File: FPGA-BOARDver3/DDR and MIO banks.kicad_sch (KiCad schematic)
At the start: 1 part, among them U1 XC7Z020-1CLG400I__

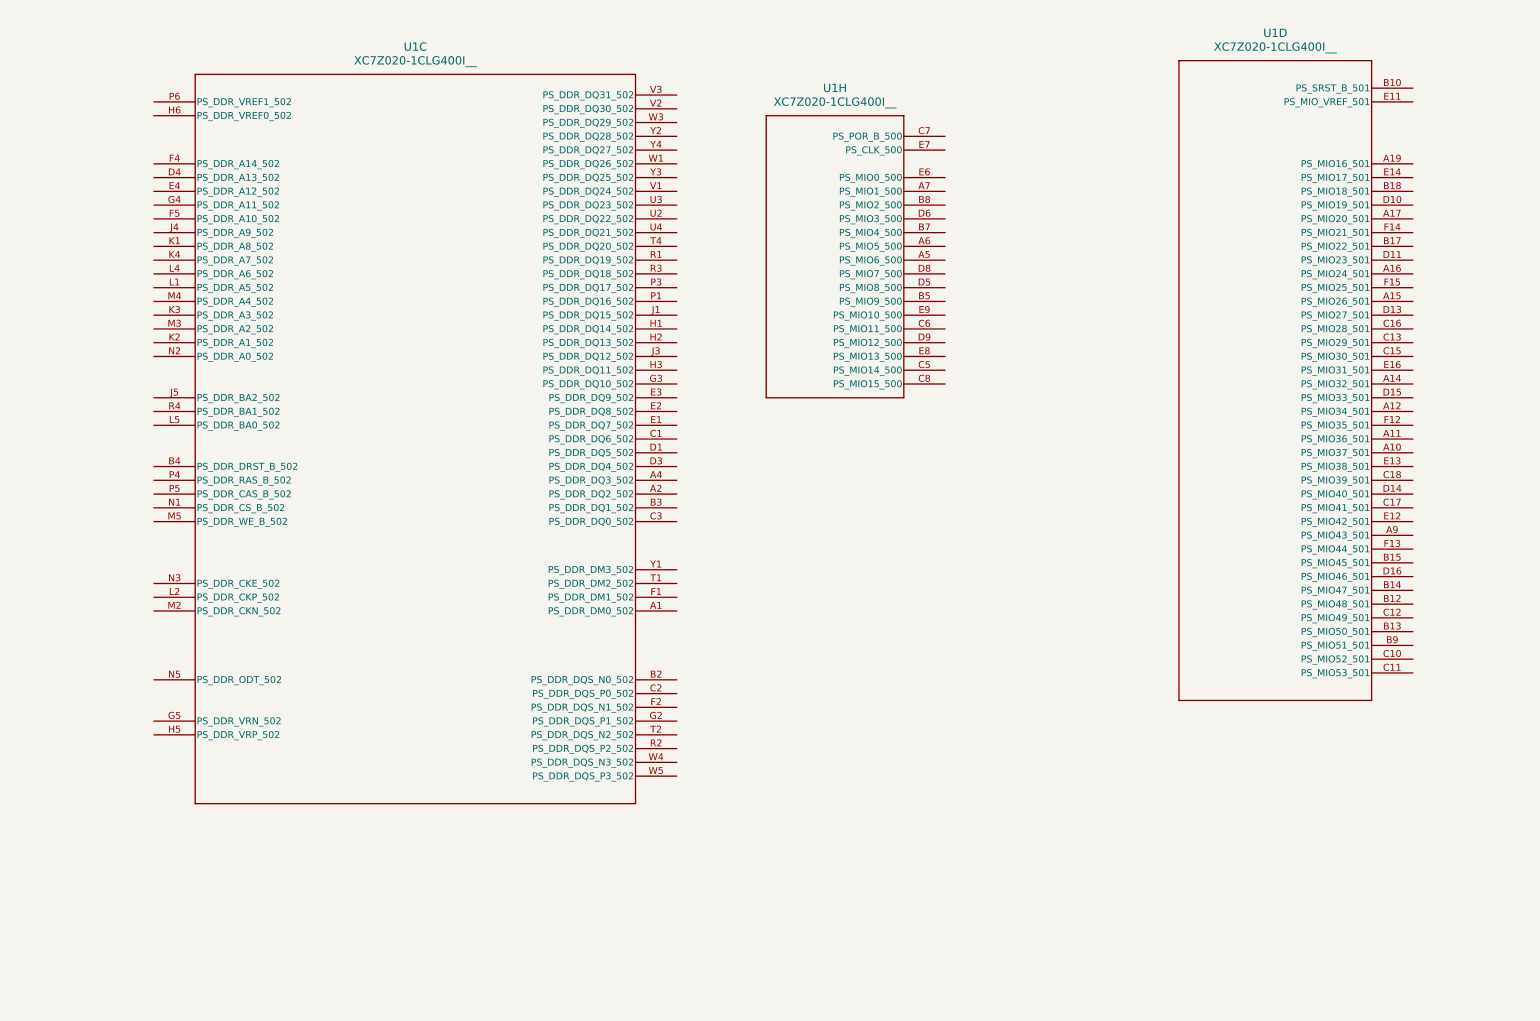
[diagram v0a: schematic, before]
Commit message: spdif fpga bansks
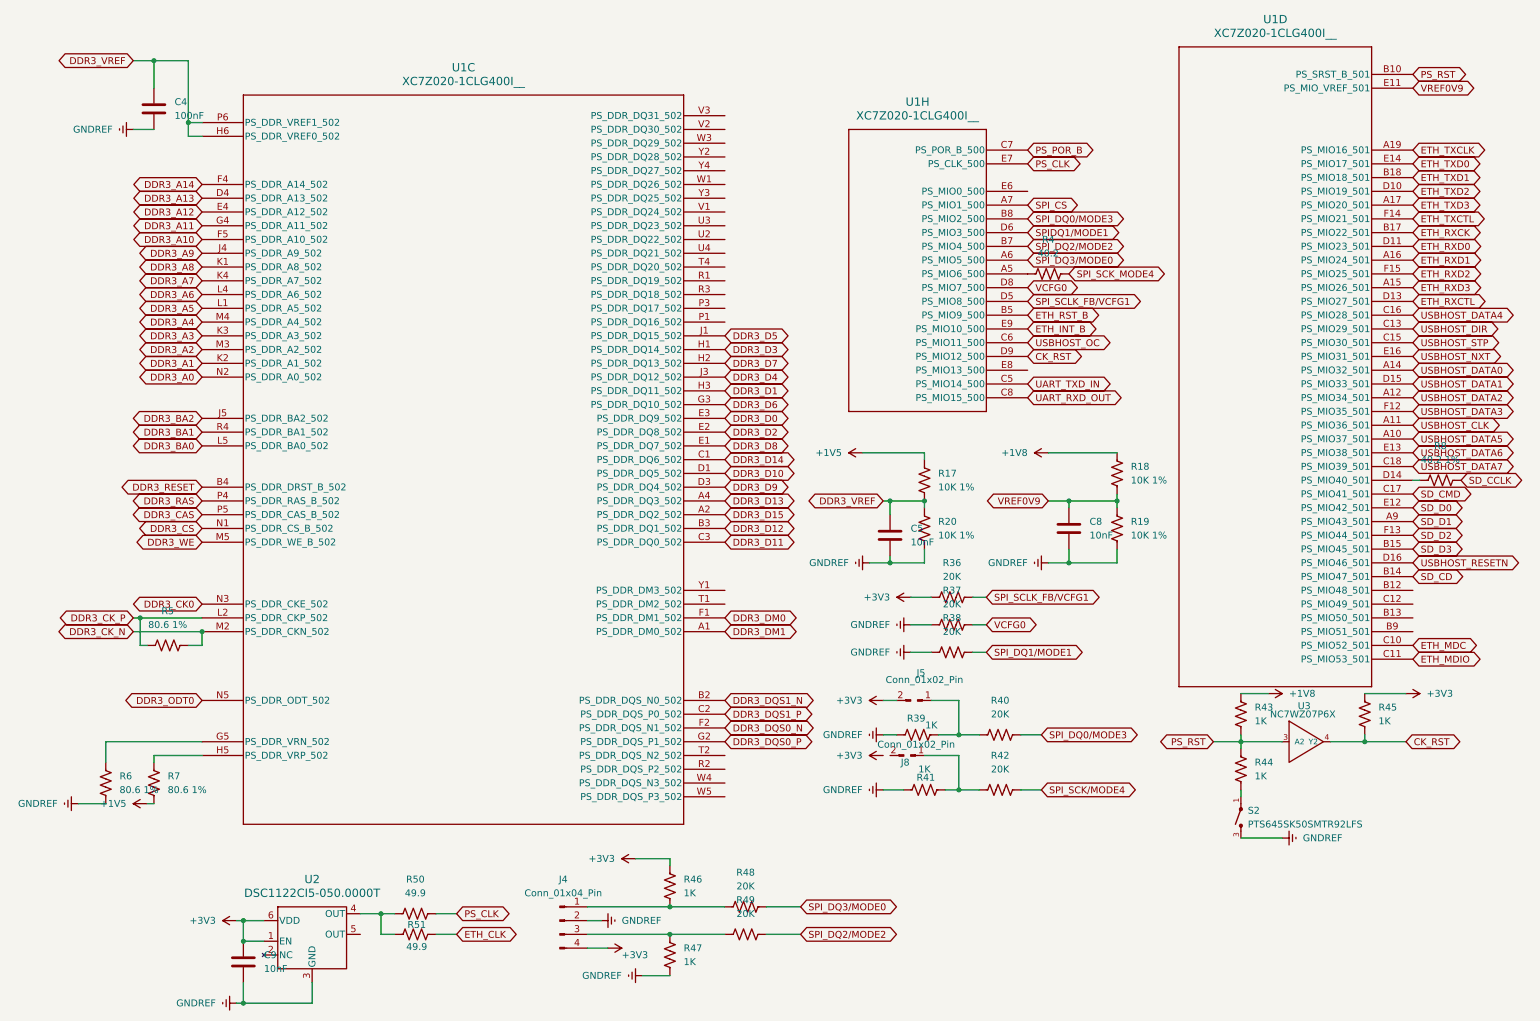
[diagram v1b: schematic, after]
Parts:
- added C4: 100nF, footprints:C_0402, symbol Device:C
- added C5, C8, C9: 10nF, footprints:C_0402, symbol Device:C
- added J4: Conn_01x04_Pin, footprints:CONN_PZ254V-11-04P_XFC, symbol Connector:Conn_01x04_Pin
- added J5, J8: Conn_01x02_Pin, footprints:CONN_PZ254V-11-02P_02P_XFC, symbol Connector:Conn_01x02_Pin
- added R17, R18, R19, R20: 10K 1%, footprints:R_0402, symbol Device:R_US
- added R36, R37, R38, R40, R42, R48, R49: 20K, footprints:R_0402, symbol Device:R_US
- added R39, R41, R43, R44, R45, R46, R47: 1K, footprints:R_0402, symbol Device:R_US
- added R4: 40.2, footprints:R_0402, symbol Device:R_US
- added R5, R6, R7: 80.6 1%, footprints:R_0402, symbol Device:R_US
- added R50, R51: 49.9, footprints:R_0402, symbol Device:R_US
- added R8: 40.2 1%, footprints:R_0402, symbol Device:R_US
- added S2: PTS645SK50SMTR92LFS, footprints:SW_PTS645SK50SMTR92LFS, symbol PTS645SK50SMTR92LFS:PTS645SK50SMTR92LFS
- added U2: DSC1122CI5-050.0000T, footprints:VDFN6_3P2X2P5_MCH, symbol 2025-04-06_19-32-54:DSC1122CI5-050.0000T
- added U3: NC7WZ07P6X, footprints:NC7WZ07P6X, symbol NC7WZ07P6X:NC7WZ07P6X
- U1: footprint footprints:CLG400_ZYNQ-7000_AMD -> XC7Z020-1CLG400I:CLG400_ZYNQ-7000_AMD
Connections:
- net DDR3_DM1: now reaches U1.A1 (PS_DDR_DM0_502)
- net DDR3_D15: now reaches U1.A2 (PS_DDR_DQ2_502)
- net DDR3_D13: now reaches U1.A4 (PS_DDR_DQ3_502)
- net DDR3_DQS1_N: now reaches U1.B2 (PS_DDR_DQS_N0_502)
- net DDR3_D12: now reaches U1.B3 (PS_DDR_DQ1_502)
- net DDR3_RESET: now reaches U1.B4 (PS_DDR_DRST_B_502)
- net DDR3_D14: now reaches U1.C1 (PS_DDR_DQ6_502)
- net DDR3_DQS1_P: now reaches U1.C2 (PS_DDR_DQS_P0_502)
- net DDR3_D11: now reaches U1.C3 (PS_DDR_DQ0_502)
- net DDR3_D10: now reaches U1.D1 (PS_DDR_DQ5_502)
- net DDR3_D9: now reaches U1.D3 (PS_DDR_DQ4_502)
- net DDR3_A13: now reaches U1.D4 (PS_DDR_A13_502)
- net DDR3_D8: now reaches U1.E1 (PS_DDR_DQ7_502)
- net DDR3_D2: now reaches U1.E2 (PS_DDR_DQ8_502)
- net DDR3_D0: now reaches U1.E3 (PS_DDR_DQ9_502)
- net DDR3_A12: now reaches U1.E4 (PS_DDR_A12_502)
- net DDR3_DM0: now reaches U1.F1 (PS_DDR_DM1_502)
- net DDR3_DQS0_N: now reaches U1.F2 (PS_DDR_DQS_N1_502)
- net DDR3_A14: now reaches U1.F4 (PS_DDR_A14_502)
- net DDR3_A10: now reaches U1.F5 (PS_DDR_A10_502)
- net DDR3_DQS0_P: now reaches U1.G2 (PS_DDR_DQS_P1_502)
- net DDR3_D6: now reaches U1.G3 (PS_DDR_DQ10_502)
- net DDR3_A11: now reaches U1.G4 (PS_DDR_A11_502)
- net at U1.G5 (PS_DDR_VRN_502): now also R6.2
- net DDR3_D3: now reaches U1.H1 (PS_DDR_DQ14_502)
- net DDR3_D7: now reaches U1.H2 (PS_DDR_DQ13_502)
- net DDR3_D1: now reaches U1.H3 (PS_DDR_DQ11_502)
- net at U1.H5 (PS_DDR_VRP_502): now also R7.2
- net DDR3_VREF: now reaches U1.H6 (PS_DDR_VREF0_502)
- net DDR3_VREF: now also U1.P6 (PS_DDR_VREF1_502), C4.1, C5.1, R17.2, R20.1
- net DDR3_D5: now reaches U1.J1 (PS_DDR_DQ15_502)
- net DDR3_D4: now reaches U1.J3 (PS_DDR_DQ12_502)
- net DDR3_A9: now reaches U1.J4 (PS_DDR_A9_502)
- net DDR3_BA2: now reaches U1.J5 (PS_DDR_BA2_502)
- net DDR3_A8: now reaches U1.K1 (PS_DDR_A8_502)
- net DDR3_A1: now reaches U1.K2 (PS_DDR_A1_502)
- net DDR3_A3: now reaches U1.K3 (PS_DDR_A3_502)
- net DDR3_A7: now reaches U1.K4 (PS_DDR_A7_502)
- net DDR3_A5: now reaches U1.L1 (PS_DDR_A5_502)
- net DDR3_CK_P: now reaches U1.L2 (PS_DDR_CKP_502)
- net DDR3_CK_P: now also R5.1
- net DDR3_A6: now reaches U1.L4 (PS_DDR_A6_502)
- net DDR3_BA0: now reaches U1.L5 (PS_DDR_BA0_502)
- net DDR3_CK_N: now reaches U1.M2 (PS_DDR_CKN_502)
- net DDR3_CK_N: now also R5.2
- net DDR3_A2: now reaches U1.M3 (PS_DDR_A2_502)
- net DDR3_A4: now reaches U1.M4 (PS_DDR_A4_502)
- net DDR3_WE: now reaches U1.M5 (PS_DDR_WE_B_502)
- net DDR3_CS: now reaches U1.N1 (PS_DDR_CS_B_502)
- net DDR3_A0: now reaches U1.N2 (PS_DDR_A0_502)
- net DDR3_CK0: now reaches U1.N3 (PS_DDR_CKE_502)
- net DDR3_ODT0: now reaches U1.N5 (PS_DDR_ODT_502)
- net DDR3_RAS: now reaches U1.P4 (PS_DDR_RAS_B_502)
- net DDR3_CAS: now reaches U1.P5 (PS_DDR_CAS_B_502)
- net DDR3_BA1: now reaches U1.R4 (PS_DDR_BA1_502)
- net USBHOST_DATA5: now reaches U1.A10 (PS_MIO37_501)
- net USBHOST_CLK: now reaches U1.A11 (PS_MIO36_501)
- net USBHOST_DATA2: now reaches U1.A12 (PS_MIO34_501)
- net USBHOST_DATA0: now reaches U1.A14 (PS_MIO32_501)
- net ETH_RXD3: now reaches U1.A15 (PS_MIO26_501)
- net ETH_RXD1: now reaches U1.A16 (PS_MIO24_501)
- net ETH_TXD3: now reaches U1.A17 (PS_MIO20_501)
- net ETH_TXCLK: now reaches U1.A19 (PS_MIO16_501)
- net SD_D1: now reaches U1.A9 (PS_MIO43_501)
- net PS_RST: now reaches U1.B10 (PS_SRST_B_501)
- net PS_RST: now also R43.2, R44.2, U3.3 (A2)
- net SD_CD: now reaches U1.B14 (PS_MIO47_501)
- net SD_D3: now reaches U1.B15 (PS_MIO45_501)
- net ETH_RXCK: now reaches U1.B17 (PS_MIO22_501)
- net ETH_TXD1: now reaches U1.B18 (PS_MIO18_501)
- net ETH_MDC: now reaches U1.C10 (PS_MIO52_501)
- net ETH_MDIO: now reaches U1.C11 (PS_MIO53_501)
- net USBHOST_DIR: now reaches U1.C13 (PS_MIO29_501)
- net USBHOST_STP: now reaches U1.C15 (PS_MIO30_501)
- net USBHOST_DATA4: now reaches U1.C16 (PS_MIO28_501)
- net SD_CMD: now reaches U1.C17 (PS_MIO41_501)
- net USBHOST_DATA7: now reaches U1.C18 (PS_MIO39_501)
- net ETH_TXD2: now reaches U1.D10 (PS_MIO19_501)
- net ETH_RXD0: now reaches U1.D11 (PS_MIO23_501)
- net ETH_RXCTL: now reaches U1.D13 (PS_MIO27_501)
- net at U1.D14 (PS_MIO40_501): now also R8.1
- net USBHOST_DATA1: now reaches U1.D15 (PS_MIO33_501)
- net USBHOST_RESETN: now reaches U1.D16 (PS_MIO46_501)
- net VREF0V9: now reaches U1.E11 (PS_MIO_VREF_501)
- net VREF0V9: now also C8.1, R18.2, R19.1
- net SD_D0: now reaches U1.E12 (PS_MIO42_501)
- net USBHOST_DATA6: now reaches U1.E13 (PS_MIO38_501)
- net ETH_TXD0: now reaches U1.E14 (PS_MIO17_501)
- net USBHOST_NXT: now reaches U1.E16 (PS_MIO31_501)
- net USBHOST_DATA3: now reaches U1.F12 (PS_MIO35_501)
- net SD_D2: now reaches U1.F13 (PS_MIO44_501)
- net ETH_TXCTL: now reaches U1.F14 (PS_MIO21_501)
- net ETH_RXD2: now reaches U1.F15 (PS_MIO25_501)
- net at U1.A5 (PS_MIO6_500): now also R4.1
- net SPI_DQ3/MODE0: now reaches U1.A6 (PS_MIO5_500)
- net SPI_DQ3/MODE0: now also R48.1
- net SPI_CS: now reaches U1.A7 (PS_MIO1_500)
- net ETH_RST_B: now reaches U1.B5 (PS_MIO9_500)
- net SPI_DQ2/MODE2: now reaches U1.B7 (PS_MIO4_500)
- net SPI_DQ2/MODE2: now also R49.1
- net SPI_DQ0/MODE3: now reaches U1.B8 (PS_MIO2_500)
- net SPI_DQ0/MODE3: now also R40.2
- net UART_TXD_IN: now reaches U1.C5 (PS_MIO14_500)
- net USBHOST_OC: now reaches U1.C6 (PS_MIO11_500)
- net PS_POR_B: now reaches U1.C7 (PS_POR_B_500)
- net UART_RXD_OUT: now reaches U1.C8 (PS_MIO15_500)
- net SPI_SCLK_FB/VCFG1: now reaches U1.D5 (PS_MIO8_500)
- net SPI_SCLK_FB/VCFG1: now also R36.2
- net SPIDQ1/MODE1: now reaches U1.D6 (PS_MIO3_500)
- net VCFG0: now reaches U1.D8 (PS_MIO7_500)
- net VCFG0: now also R37.2
- net CK_RST: now reaches U1.D9 (PS_MIO12_500)
- net CK_RST: now also R45.1, U3.4 (Y2)
- net PS_CLK: now reaches U1.E7 (PS_CLK_500)
- net PS_CLK: now also R50.1
- net ETH_INT_B: now reaches U1.E9 (PS_MIO10_500)
- new net: J4.3 (Pin_3), R47.2, R49.2
- new net: J8.1 (Pin_1), R41.2, R42.1
- new net: R50.2, R51.2, U2.4 (OUT)
- new net: J4.1 (Pin_1), R46.1, R48.2
- new net: R44.1, S2.1
- new net: J5.1 (Pin_1), R39.2, R40.1
- new net +1V5: R17.1, R7.1
- new net +1V8: R18.1, R43.1
- new net +3V3: C9.1, J4.4 (Pin_4), J5.2 (Pin_2), R36.1, R45.2, R46.2, U2.1 (EN), U2.6 (VDD)
- new net ETH_CLK: R51.1
- new net GNDREF: C4.2, C5.2, C8.2, C9.2, J4.2 (Pin_2), R19.2, R20.2, R37.1, R38.1, R39.1, R41.1, R47.1, R6.1, S2.3, U2.3 (GND)
- new net SD_CCLK: R8.2
- new net SPI_DQ1/MODE1: R38.2
- new net SPI_SCK_MODE4: R4.2
- new net SPI_SCK/MODE4: R42.2
